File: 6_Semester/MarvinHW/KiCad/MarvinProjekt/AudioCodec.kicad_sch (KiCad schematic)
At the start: 51 parts, among them U2 ES8388, U3 MP1720

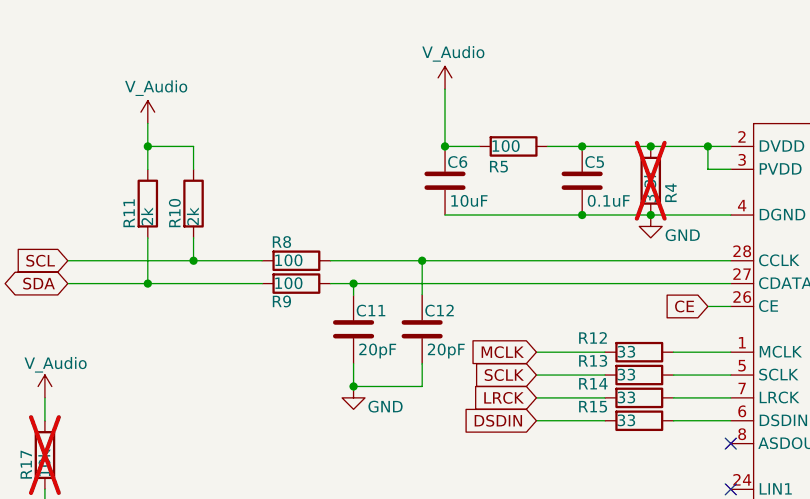
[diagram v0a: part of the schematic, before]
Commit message: finish evaluat components
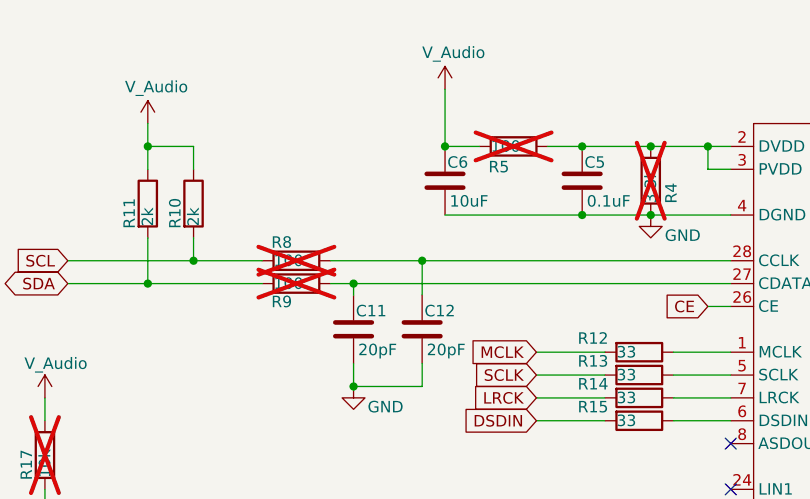
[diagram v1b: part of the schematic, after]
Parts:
- R5, R8, R9: now not fitted
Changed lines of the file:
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@@
 		(in_bom yes)
 		(on_board yes)
-		(dnp no)
+		(dnp yes)
 		(property "Reference" "R9"
 			(at 45.466 43.942 90)
@@
 		(in_bom yes)
 		(on_board yes)
-		(dnp no)
+		(dnp yes)
 		(property "Reference" "R8"
 			(at 45.466 37.338 90)
@@
 		(in_bom yes)
 		(on_board yes)
-		(dnp no)
+		(dnp yes)
 		(property "Reference" "R5"
 			(at 69.596 28.956 90)
